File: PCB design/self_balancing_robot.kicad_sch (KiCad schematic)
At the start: 29 parts, among them J1 I2C, J2 Conn_01x06_Socket, J3 Conn_01x02_Socket, J4 Conn_01x04_Socket, J6 SPI, J7 Conn_01x04_Pin, SW1 SW_Push, U1 ATmega328P-A, U2 L293D, U4 LP2985-3.3, U5 NCP1117-5.0_SOT223, Y1 Crystal

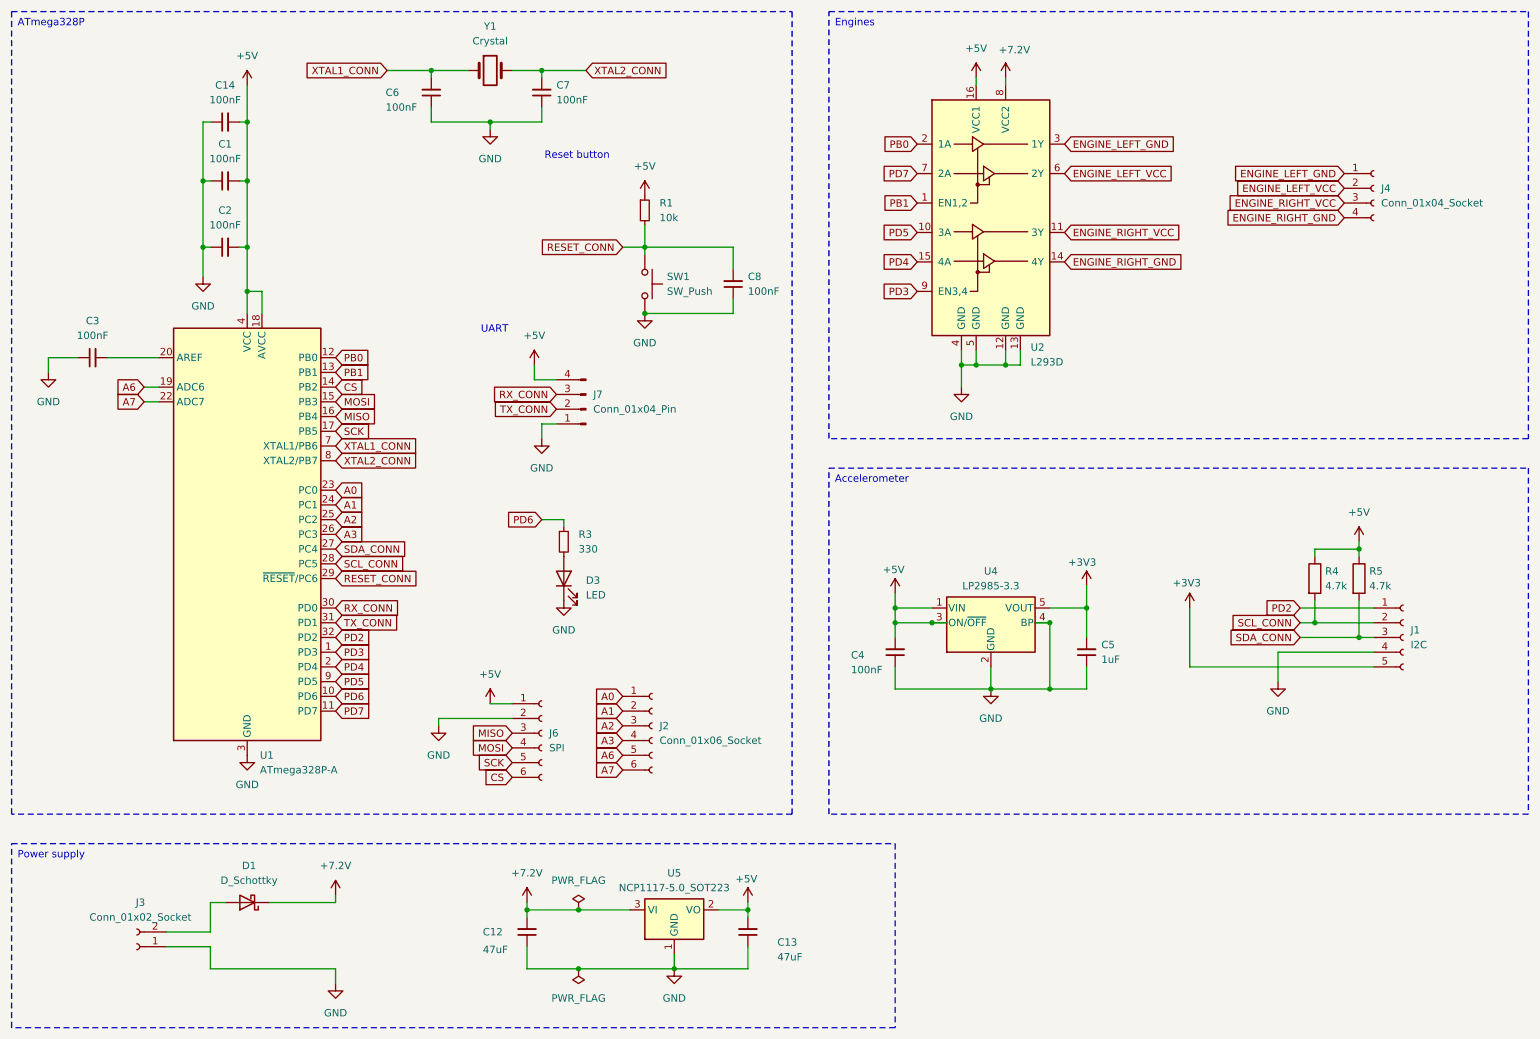
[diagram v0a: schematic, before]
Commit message: PCB update - almost finishing
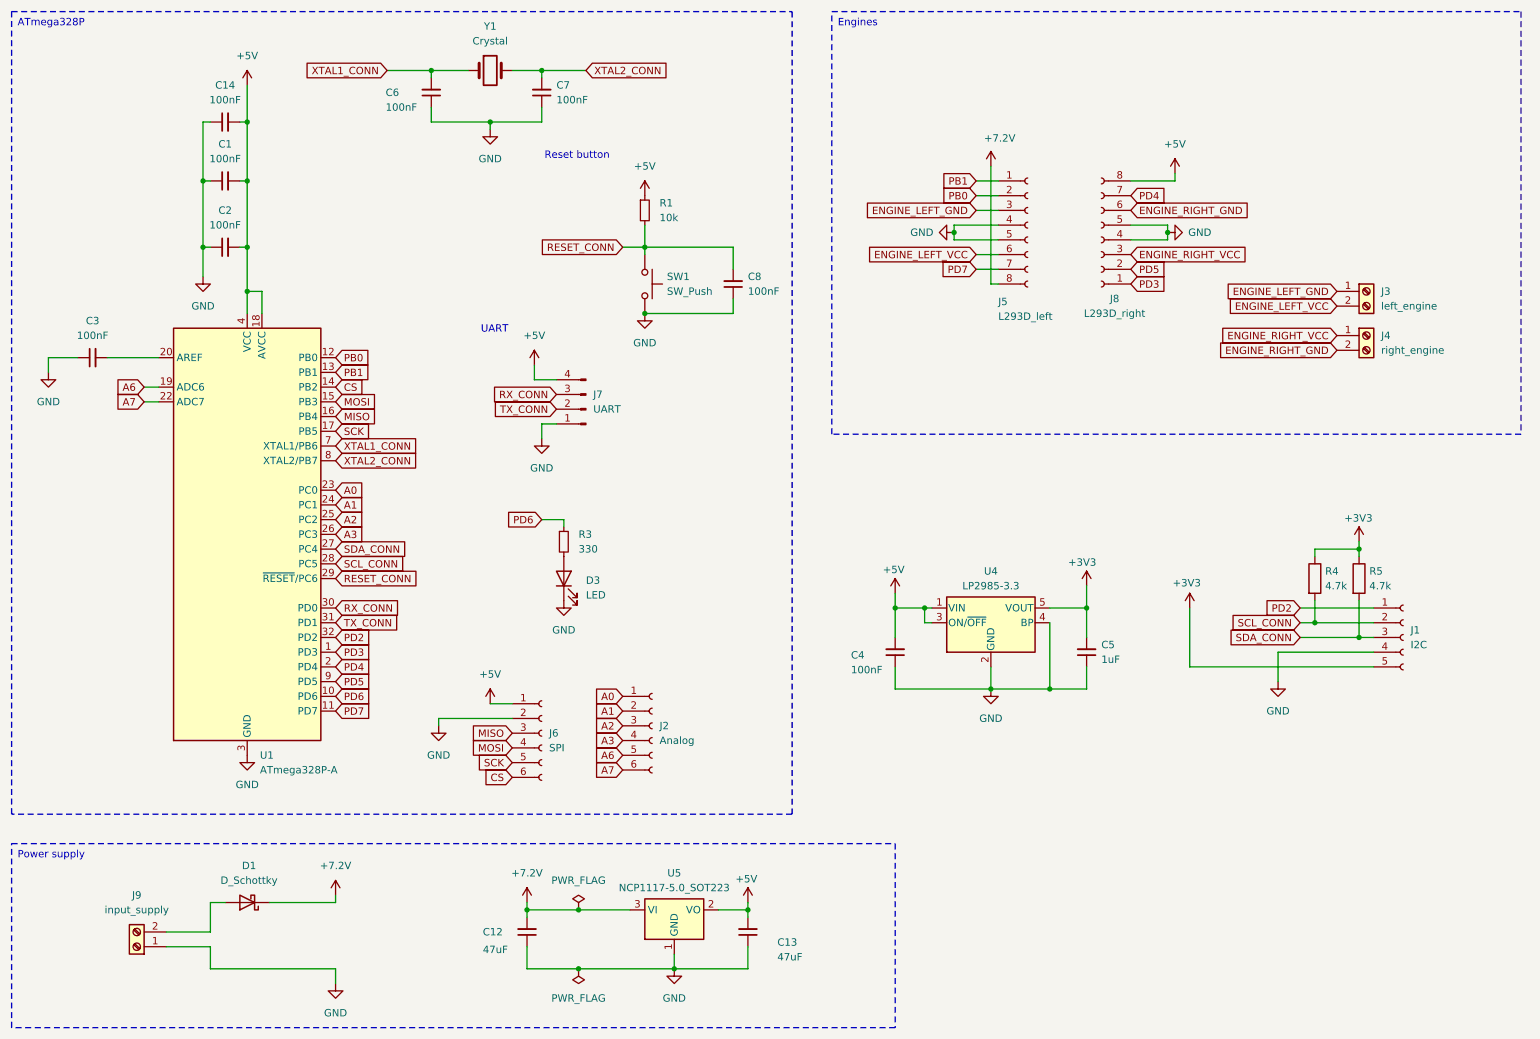
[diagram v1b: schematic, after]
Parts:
- removed J3: Conn_01x02_Socket, Connector_PinSocket_2.54mm:PinSocket_1x02_P2.54mm_Vertical, symbol Connector:Conn_01x02_Socket
- removed J4: Conn_01x04_Socket, Connector_PinSocket_2.54mm:PinSocket_1x04_P2.54mm_Vertical, symbol Connector:Conn_01x04_Socket
- removed U2: L293D, Package_DIP:DIP-16_W7.62mm, symbol Driver_Motor:L293D
- added J3: left_engine, Connector_TE-Connectivity:TE_826576-2_1x02_P3.96mm_Vertical, symbol Connector:Screw_Terminal_01x02
- added J4: right_engine, Connector_TE-Connectivity:TE_826576-2_1x02_P3.96mm_Vertical, symbol Connector:Screw_Terminal_01x02
- added J5: L293D_left, Connector_PinSocket_2.54mm:PinSocket_1x08_P2.54mm_Vertical, symbol Connector:Conn_01x08_Socket
- added J8: L293D_right, Connector_PinSocket_2.54mm:PinSocket_1x08_P2.54mm_Vertical, symbol Connector:Conn_01x08_Socket
- added J9: input_supply, Connector_TE-Connectivity:TE_826576-2_1x02_P3.96mm_Vertical, symbol Connector:Screw_Terminal_01x02
- C1, C12, C13, C14, C2, C3, C4, C5, C6, C7, C8: footprint Capacitor_THT:C_Disc_D5.0mm_W2.5mm_P2.50mm -> Capacitor_SMD:C_0805_2012Metric
- D1: footprint Resistor_THT:R_Axial_DIN0204_L3.6mm_D1.6mm_P5.08mm_Horizontal -> Resistor_THT:R_Axial_DIN0207_L6.3mm_D2.5mm_P7.62mm_Horizontal
- J2: value Conn_01x06_Socket -> Analog
- J7: value Conn_01x04_Pin -> UART
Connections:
- net +3V3: now also R4.1, R5.1
- net +5V: now also J8.8 (Pin_8); no longer R4.1, R5.1
- net +7.2V: now also J5.8 (Pin_8)
- net ENGINE_LEFT_GND: now also J3.1 (Pin_1), J5.3 (Pin_3)
- net ENGINE_LEFT_VCC: now also J3.2 (Pin_2), J5.6 (Pin_6)
- net ENGINE_RIGHT_GND: now also J4.2 (Pin_2), J8.6 (Pin_6)
- net ENGINE_RIGHT_VCC: now also J4.1 (Pin_1), J8.3 (Pin_3)
- net GND: now also J5.4 (Pin_4), J5.5 (Pin_5), J8.4 (Pin_4), J8.5 (Pin_5), J9.1 (Pin_1)
- net PB0: now also J5.2 (Pin_2)
- net PB1: now also J5.1 (Pin_1)
- net PD3: now also J8.1 (Pin_1)
- net PD4: now also J8.7 (Pin_7)
- net PD5: now also J8.2 (Pin_2)
- net PD7: now also J5.7 (Pin_7)
- net at D1.2 (A): now also J9.2 (Pin_2)
